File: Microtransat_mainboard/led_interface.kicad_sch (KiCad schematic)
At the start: 12 parts, among them J201 Conn_01x07

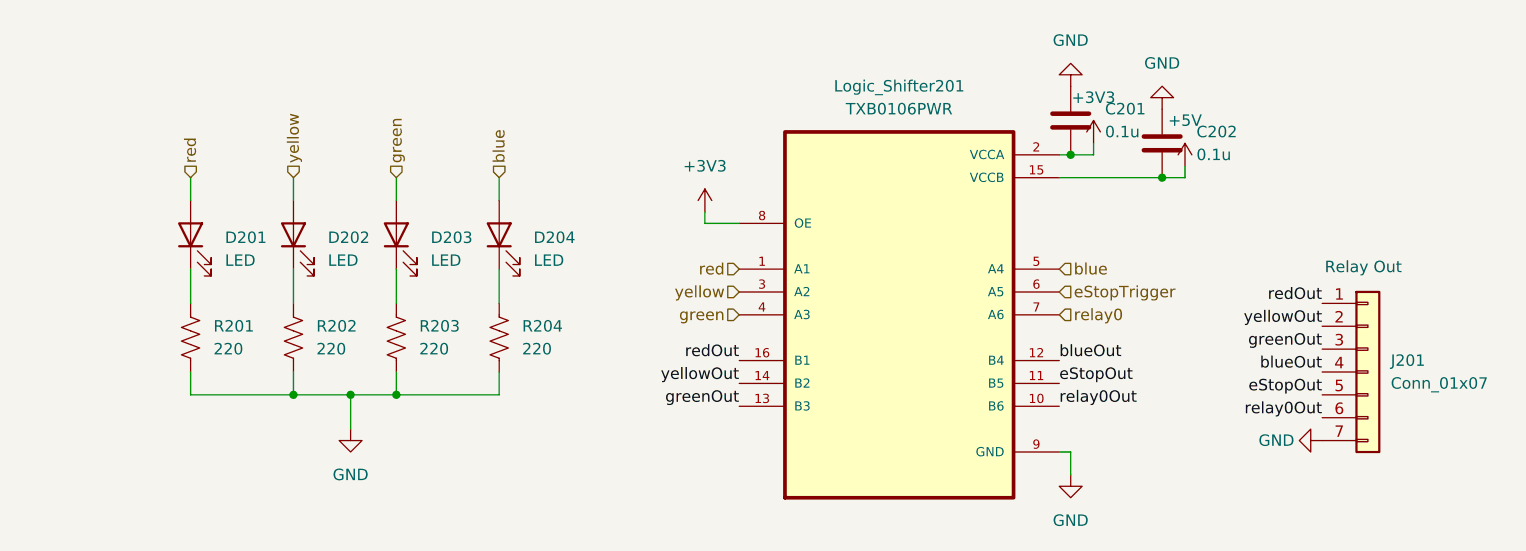
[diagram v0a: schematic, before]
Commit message: Fixed changes from design review
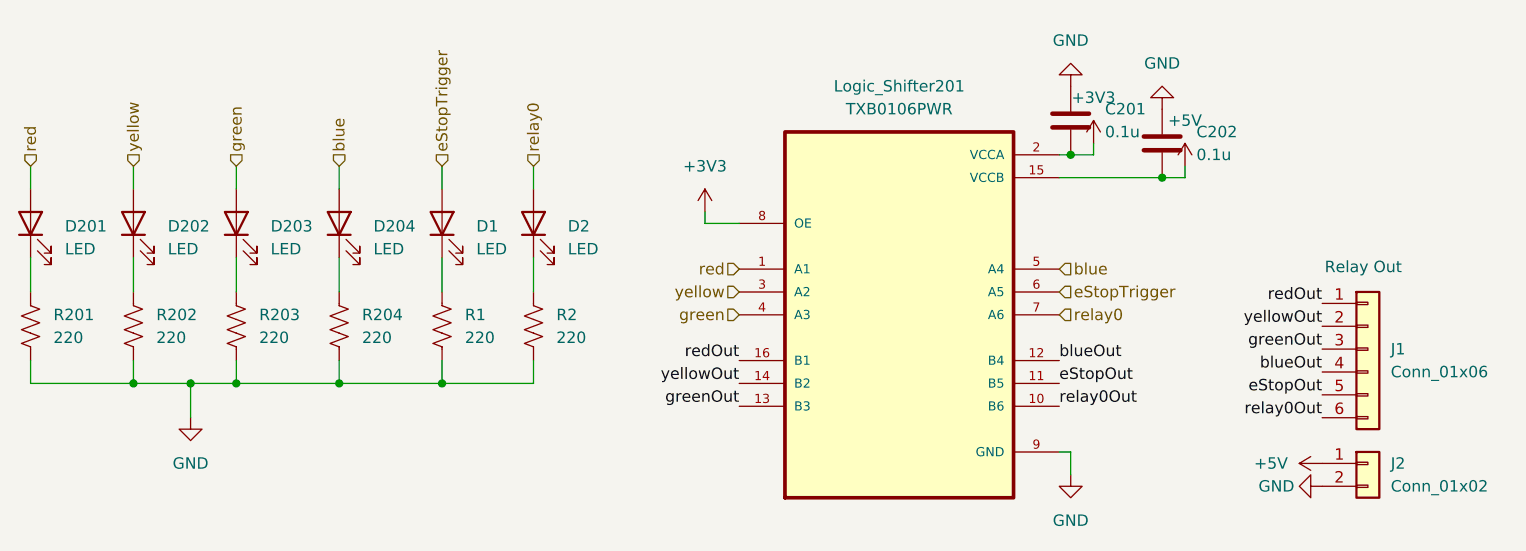
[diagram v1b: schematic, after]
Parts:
- removed J201: Conn_01x07, Connector_PinSocket_2.54mm:PinSocket_1x07_P2.54mm_Vertical, symbol Connector_Generic:Conn_01x07
- added D1, D2: LED, LED_SMD:LED_1206_3216Metric_Pad1.42x1.75mm_HandSolder, symbol Device:LED
- added J1: Conn_01x06, Connector_JST:JST_XH_B6B-XH-A_1x06_P2.50mm_Vertical, symbol Connector_Generic:Conn_01x06
- added J2: Conn_01x02, Connector_JST:JST_XH_B2B-XH-A_1x02_P2.50mm_Vertical, symbol Connector_Generic:Conn_01x02
- added R1, R2: 220, Resistor_SMD:R_1206_3216Metric_Pad1.30x1.75mm_HandSolder, symbol Device:R_US
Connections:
- net +5V: now also J2.1 (Pin_1)
- net GND: now also J2.2 (Pin_2), R1.2, R2.2
- net blueOut: now also J1.4 (Pin_4)
- net eStopOut: now also J1.5 (Pin_5)
- net eStopTrigger: now also D1.2 (A)
- net greenOut: now also J1.3 (Pin_3)
- net redOut: now also J1.1 (Pin_1)
- net relay0: now also D2.2 (A)
- net relay0Out: now also J1.6 (Pin_6)
- net yellowOut: now also J1.2 (Pin_2)
- new net: D1.1 (K), R1.1
- new net: D2.1 (K), R2.1
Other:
- moved on the sheet: D201, D202, D203, D204, R201, R202, R203, R204
